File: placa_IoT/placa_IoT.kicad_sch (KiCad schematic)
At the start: 0 parts

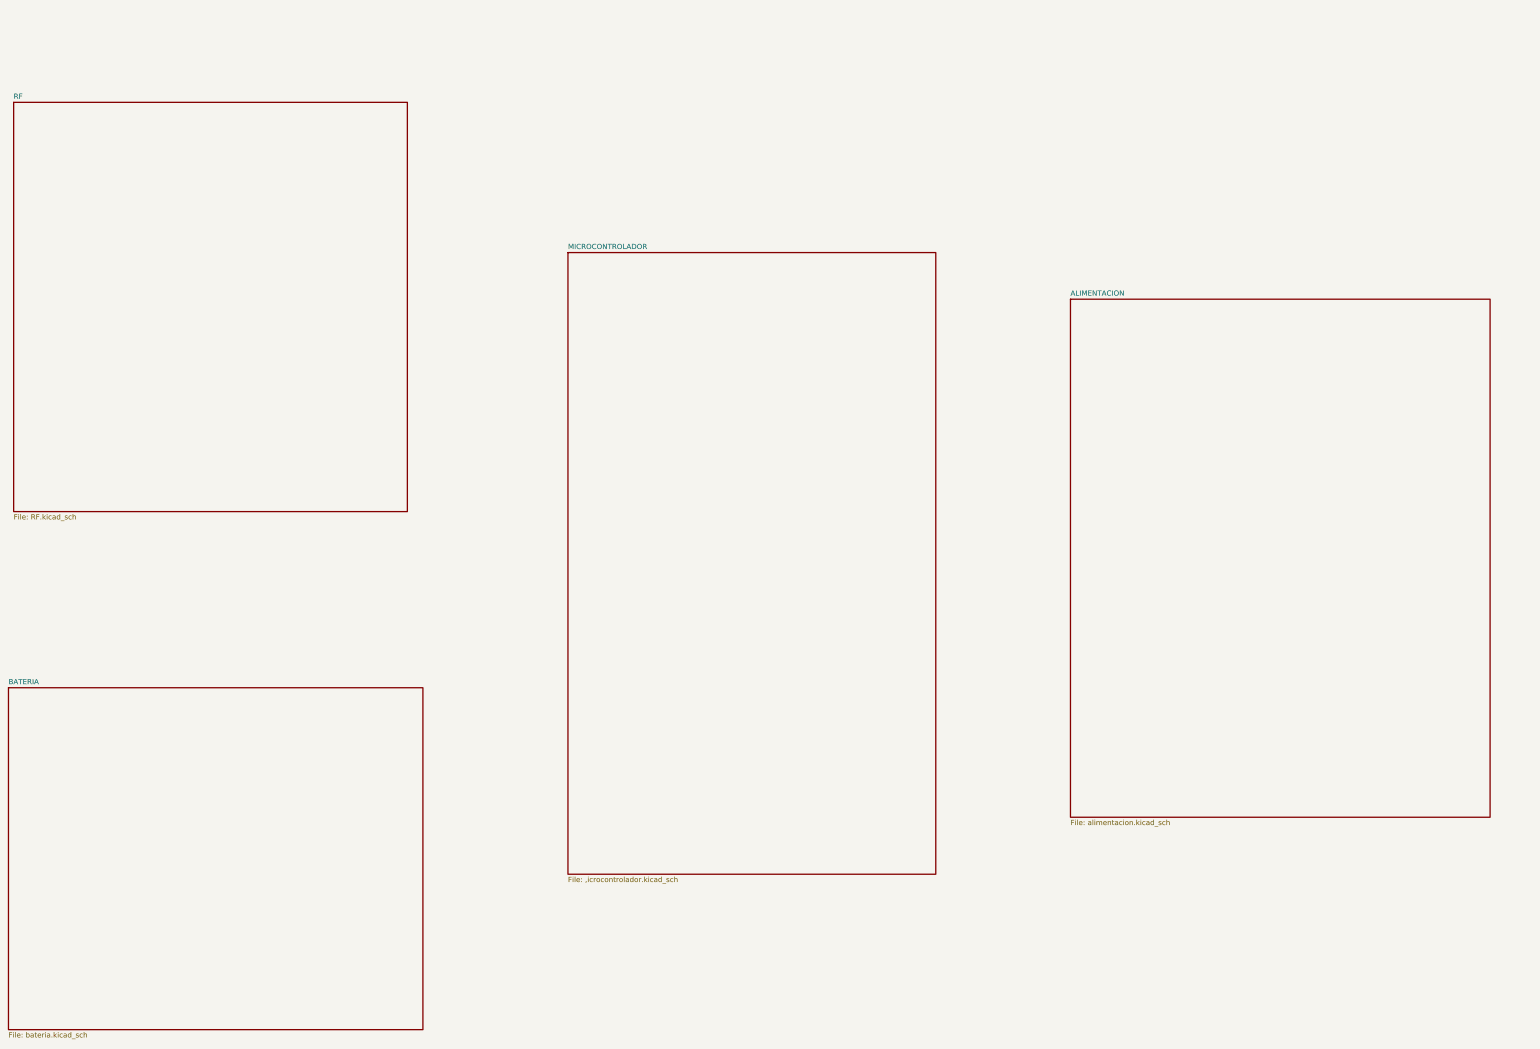
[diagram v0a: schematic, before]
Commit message: USB completed
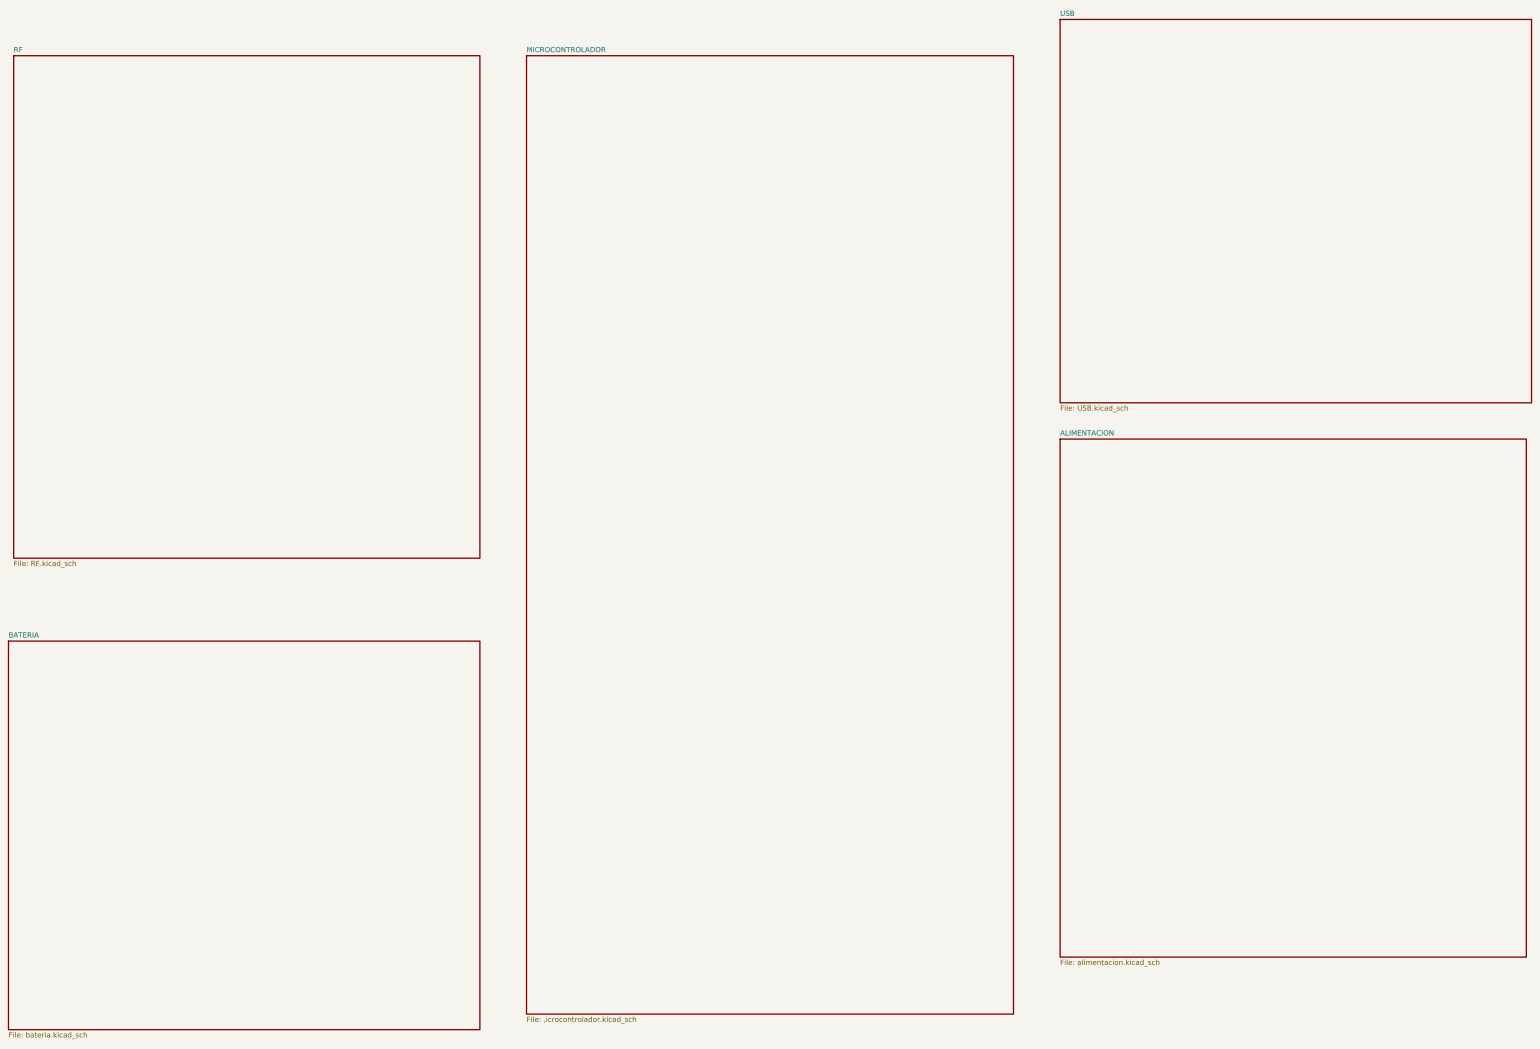
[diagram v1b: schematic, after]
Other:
- added sheet USB (USB.kicad_sch)
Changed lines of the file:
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@@
 	)
 	(sheet
-		(at 167.64 73.66)
-		(size 90.17 152.4)
+		(at 157.48 25.4)
+		(size 119.38 234.95)
 		(exclude_from_sim no)
 		(in_bom yes)
@@
 		)
 		(property "Sheetname" "MICROCONTROLADOR"
-			(at 167.64 72.9484 0)
+			(at 157.48 24.6884 0)
 			(show_name no)
 			(do_not_autoplace no)
@@
 		)
 		(property "Sheetfile" ",icrocontrolador.kicad_sch"
-			(at 167.64 226.6446 0)
+			(at 157.48 260.9346 0)
 			(show_name no)
 			(do_not_autoplace no)
@@
 	)
 	(sheet
-		(at 31.75 36.83)
-		(size 96.52 100.33)
+		(at 31.75 25.4)
+		(size 114.3 123.19)
 		(exclude_from_sim no)
 		(in_bom yes)
@@
 		)
 		(property "Sheetname" "RF"
-			(at 31.75 36.1184 0)
+			(at 31.75 24.6884 0)
 			(show_name no)
 			(do_not_autoplace no)
@@
 		)
 		(property "Sheetfile" "RF.kicad_sch"
-			(at 31.75 137.7446 0)
+			(at 31.75 149.1746 0)
 			(show_name no)
 			(do_not_autoplace no)
@@
 	)
 	(sheet
-		(at 30.48 180.34)
-		(size 101.6 83.82)
+		(at 30.48 168.91)
+		(size 115.57 95.25)
 		(exclude_from_sim no)
 		(in_bom yes)
@@
 		)
 		(property "Sheetname" "BATERIA"
-			(at 30.48 179.6284 0)
+			(at 30.48 168.1984 0)
 			(show_name no)
 			(do_not_autoplace no)
@@
 	)
 	(sheet
-		(at 290.83 85.09)
-		(size 102.87 127)
+		(at 288.29 16.51)
+		(size 115.57 93.98)
+		(exclude_from_sim no)
+		(in_bom yes)
+		(on_board yes)
+		(dnp no)
+		(fields_autoplaced yes)
+		(stroke
+			(width 0.1524)
+			(type solid)
+		)
+		(fill
+			(color 0 0 0 0)
+		)
+		(property "Sheetname" "USB"
+			(at 288.29 15.7984 0)
+			(show_name no)
+			(do_not_autoplace no)
+			(effects
+				(font
+					(size 1.27 1.27)
+				)
+				(justify left bottom)
+			)
+		)
+		(property "Sheetfile" "USB.kicad_sch"
+			(at 288.29 111.0746 0)
+			(show_name no)
+			(do_not_autoplace no)
+			(effects
+				(font
+					(size 1.27 1.27)
+				)
+				(justify left top)
+			)
+		)
+		(instances
+			(project "placa_IoT"
+				(path "/5cf00a4a-c4d0-4d7e-b436-de913efc1992"
+					(page "6")
+				)
+			)
+		)
+	)
+	(sheet
+		(at 288.29 119.38)
+		(size 114.3 127)
 		(exclude_from_sim no)
 		(in_bom yes)
@@
 		)
 		(property "Sheetname" "ALIMENTACION"
-			(at 290.83 84.3784 0)
+			(at 288.29 118.6684 0)
 			(show_name no)
 			(do_not_autoplace no)
@@
 		)
 		(property "Sheetfile" "alimentacion.kicad_sch"
-			(at 290.83 212.6746 0)
-			(show_name no)
-			(do_not_autoplace no)
+			(at 288.29 246.9646 0)
+			(show_name no)
+			(do_not_autoplace no)
